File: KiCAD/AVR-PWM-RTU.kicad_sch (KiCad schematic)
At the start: 60 parts, among them J1 12V DC, J10 Ch2, J11 Ch3, J12 Remote, J2 OUT, J3 ICSP, J4 OUT, J5 RS485, J6 OUT, J7 OUT, J8 Ch0, J9 Ch1, Q1 IRLZ44N, Q2 IRLZ44N, Q3 IRLZ44N, Q4 IRLZ44N, SW1 SW_Push, U1 L7805, U2 ATMega328-P, U3 MAX485E, U4 74HC138, Y1 8M

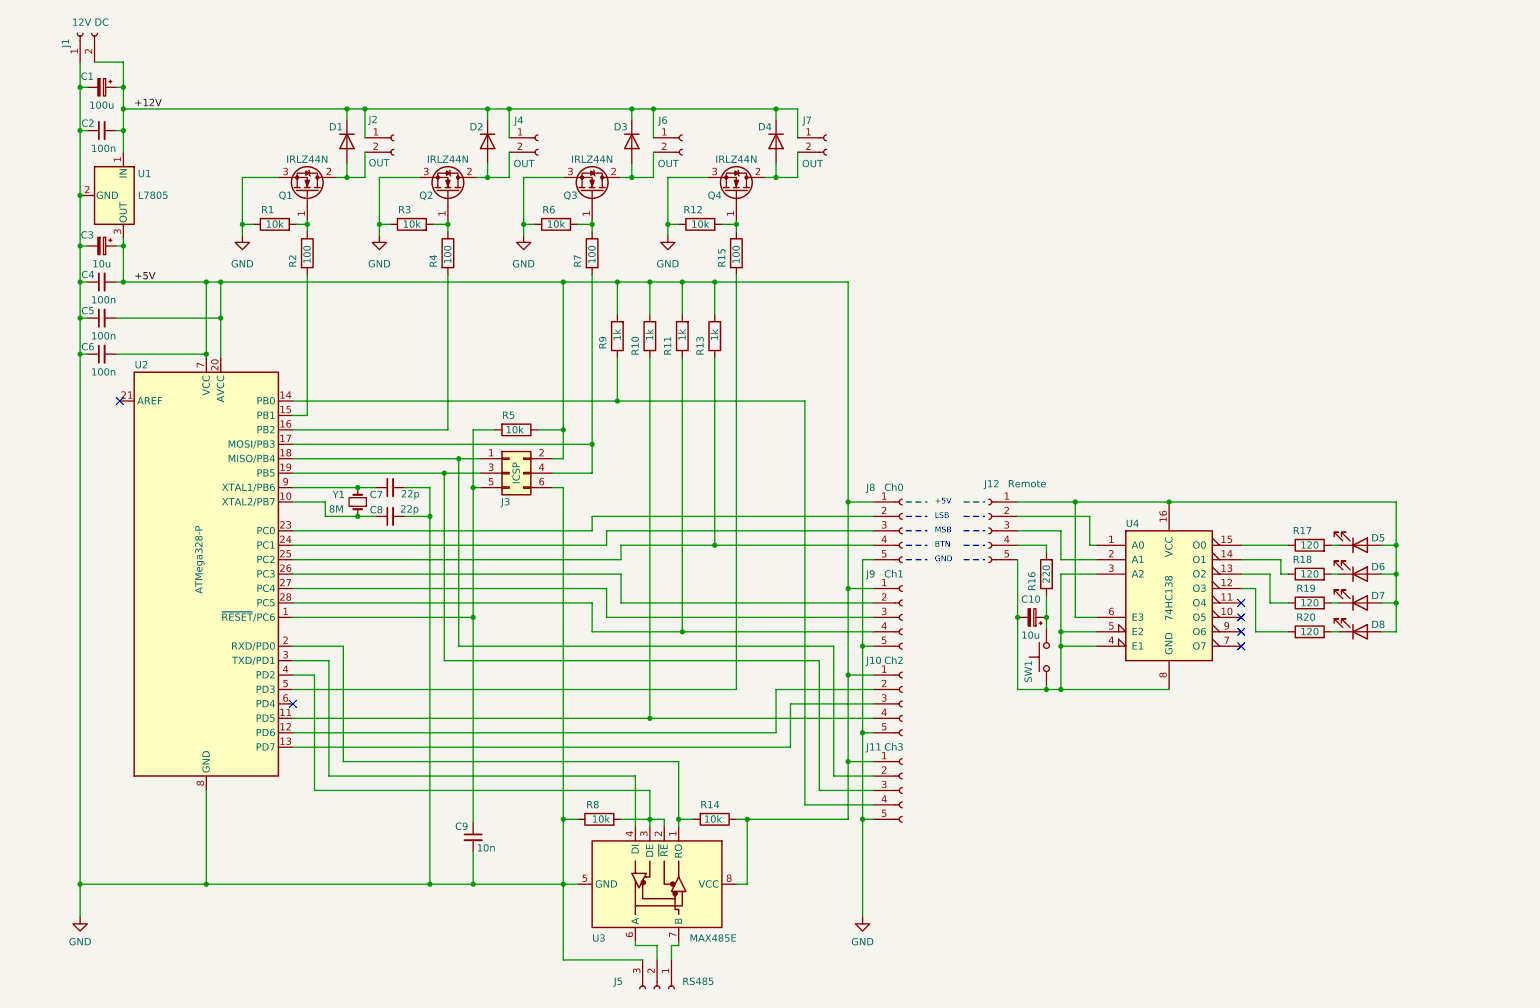
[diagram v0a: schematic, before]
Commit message: Updated schematic.
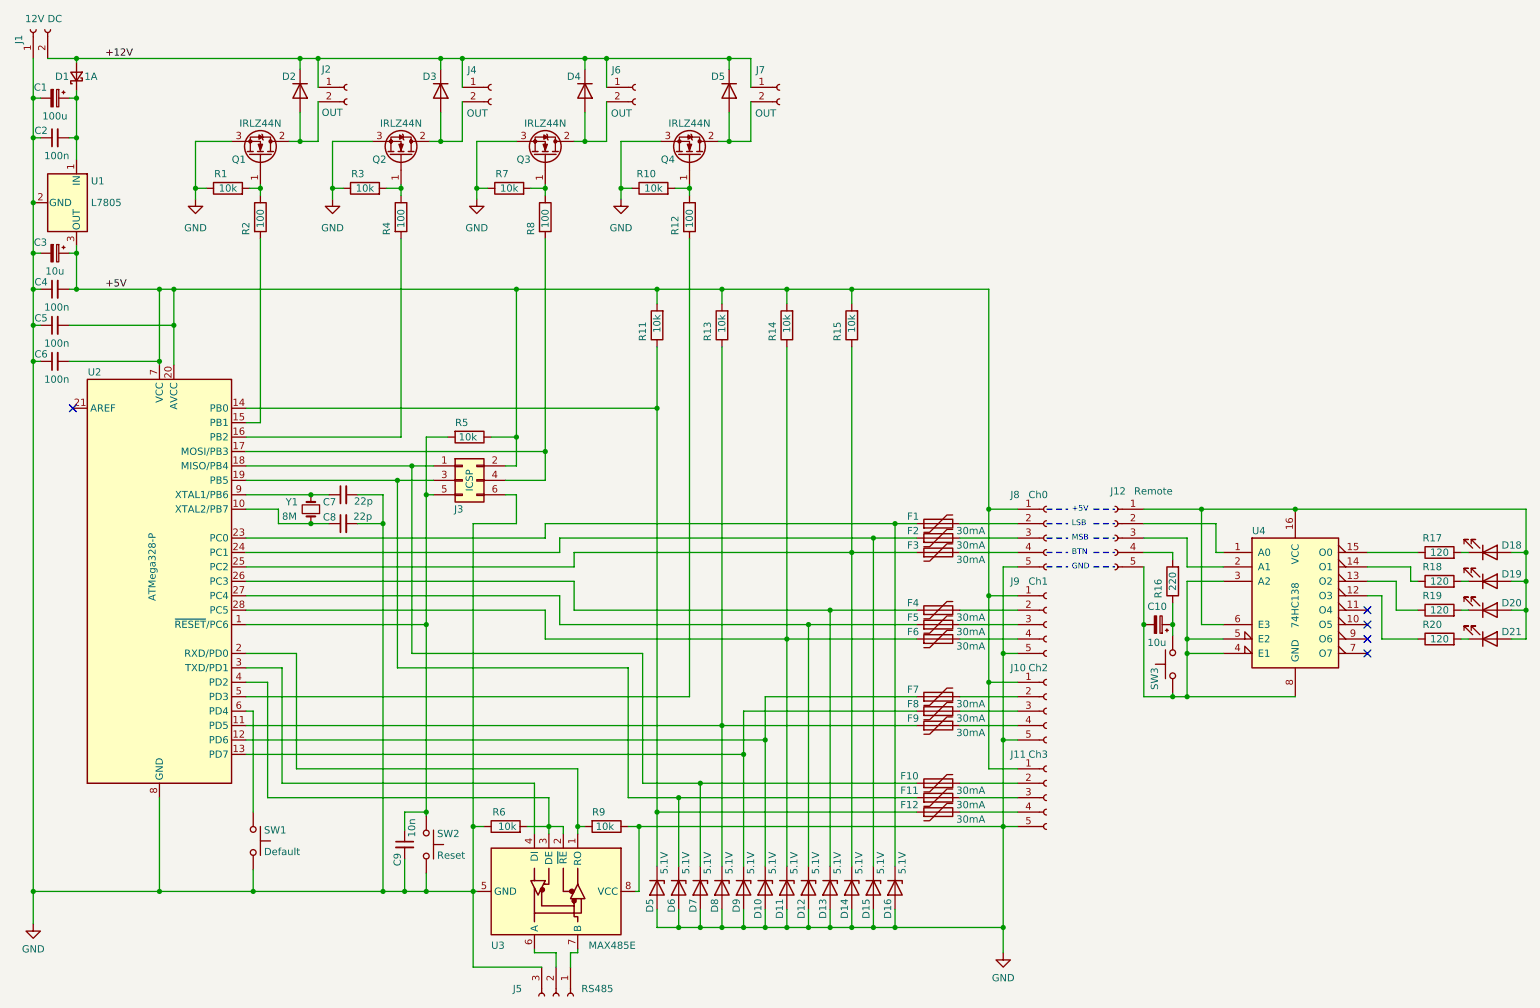
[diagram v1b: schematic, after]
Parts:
- removed R10, R11, R9: 1k, symbol Device:R
- added D1: 1A, symbol Device:D_Schottky_Small
- added D10, D11, D12, D13, D14, D15, D16, D5, D6, D7, D8, D9: 5.1V, symbol Device:D_Zener
- added F1, F10, F11, F12, F2, F3, F4, F5, F6, F7, F8, F9: 30mA, symbol Device:Polyfuse
- added R13, R14, R15: 10k, symbol Device:R
- added SW1: Default, symbol Switch:SW_Push
- added SW2: Reset, symbol Switch:SW_Push
- R11: renamed from R13; value 1k -> 10k
- U1: footprint (none) -> Package_TO_SOT_THT:TO-220-3_Vertical
- renumbered D5 to D18, D6 to D19, D1 to D2, D7 to D20, D8 to D21, D2 to D3, D3 to D4, D4 to D5, R12 to R10, R15 to R12, R8 to R6, R6 to R7, R7 to R8, R14 to R9, SW1 to SW3
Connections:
- net +12V: now also D1.2 (A); no longer C1.1, C2.2, U1.1 (IN)
- net +5V: now also R13.2, R14.2, R15.2; no longer R9.1, U3.8 (VCC)
- net GND: now also R9.1, U3.8 (VCC), D10.2 (A), D11.2 (A), D12.2 (A), D13.2 (A), D14.2 (A), D15.2 (A), D16.2 (A), D5.2 (A), D6.2 (A), D7.2 (A), D8.2 (A), D9.2 (A), SW1.2, SW2.2
- net at C9.1, J3.5 (Pin_5), R5.2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: now also SW2.1
- net at U2.11 (PD5): now also D8.1 (K), F9.1, R13.1; no longer J10.4 (Pin_4)
- net at U2.12 (PD6): now also D10.1 (K), F7.1; no longer J10.2 (Pin_2)
- net at U2.13 (PD7): now also D9.1 (K), F8.1; no longer J10.3 (Pin_3)
- net at U2.14 (PB0): now also R11.1, D5.1 (K), F12.1; no longer J11.4 (Pin_4)
- net at J3.1 (Pin_1), U2.18 (MISO/PB4): now also D7.1 (K), F10.1; no longer J11.2 (Pin_2)
- net at J3.3 (Pin_3), U2.19 (PB5): now also D6.1 (K), F11.1; no longer J11.3 (Pin_3)
- net at U2.23 (PC0): now also D16.1 (K), F1.1; no longer J8.2 (Pin_2)
- net at U2.24 (PC1): now also D15.1 (K), F2.1; no longer J8.3 (Pin_3)
- net at U2.26 (PC3): now also D13.1 (K), F4.1; no longer J9.2 (Pin_2)
- net at U2.27 (PC4): now also D12.1 (K), F5.1; no longer J9.3 (Pin_3)
- net at U2.28 (PC5): now also D11.1 (K), F6.1, R14.1; no longer J9.4 (Pin_4)
- net at U2.6 (PD4): now also SW1.1
- new net: D14.1 (K), F3.1, R15.1, U2.25 (PC2)
- new net: F11.2, J11.3 (Pin_3)
- new net: F6.2, J9.4 (Pin_4)
- new net: F1.2, J8.2 (Pin_2)
- new net: F2.2, J8.3 (Pin_3)
- new net: F3.2, J8.4 (Pin_4)
- new net: F5.2, J9.3 (Pin_3)
- new net: F12.2, J11.4 (Pin_4)
- new net: F7.2, J10.2 (Pin_2)
- new net: F8.2, J10.3 (Pin_3)
- new net: F9.2, J10.4 (Pin_4)
- new net: F4.2, J9.2 (Pin_2)
- new net: F10.2, J11.2 (Pin_2)
- new net: C1.1, C2.2, D1.1 (K), U1.1 (IN)
- no-connect marks 6 -> 5
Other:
- moved on the sheet: C1, C10, C2, C3, C4, C5, C6, C7, C8, C9, D18, D19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
